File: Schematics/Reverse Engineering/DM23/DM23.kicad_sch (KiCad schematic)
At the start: 100 parts, among them J1 Conn_01x40, Q1 2N1499A, Q2 2N1499A, Q3 2N1499A, Q4 2N1499A, Q5 2N1499A, Q6 2N1499A, Q7 2N1499A, Q8 2N1499A, Q9 2N1499A

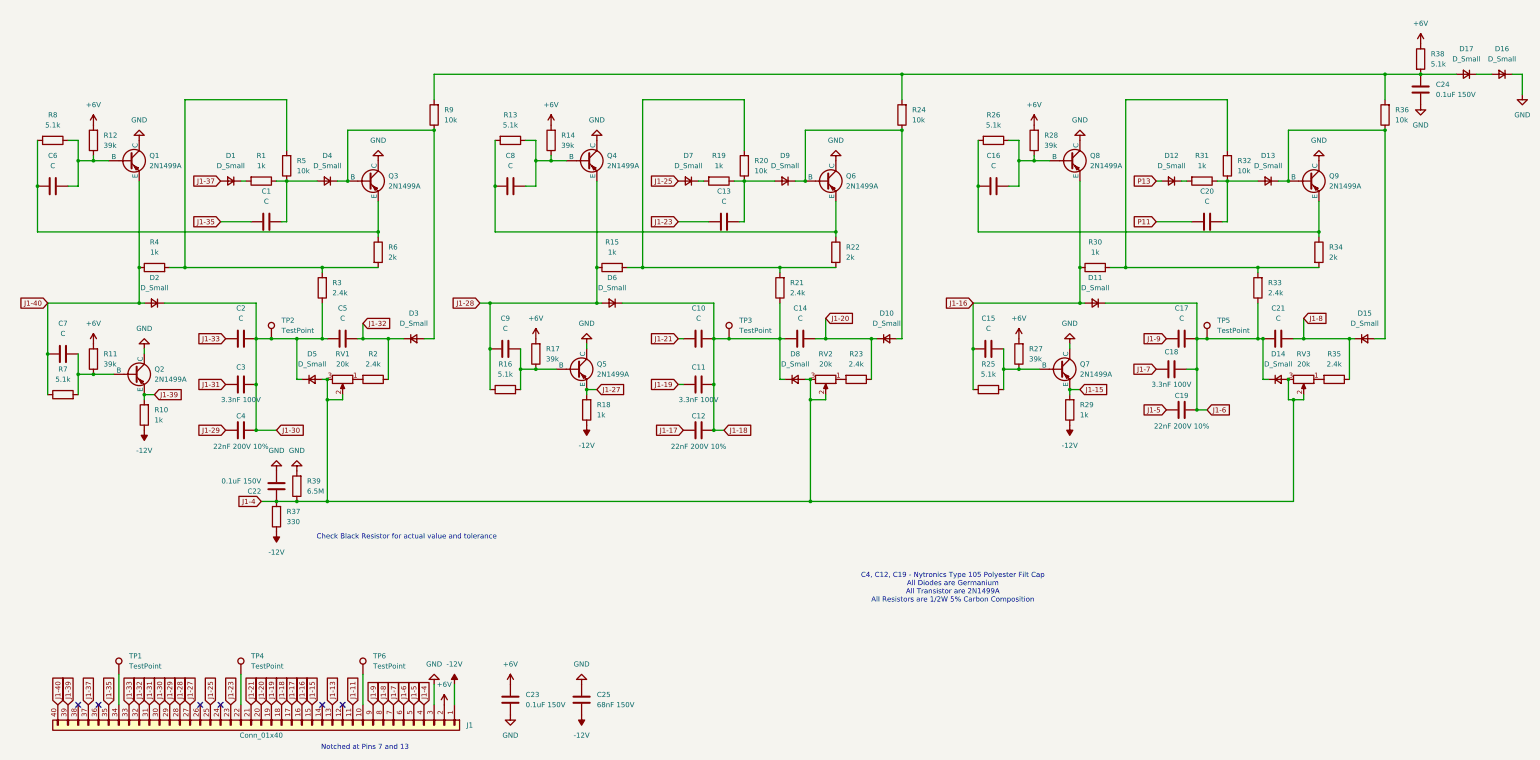
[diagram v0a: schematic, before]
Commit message: Updated Schematic Layout and PCB
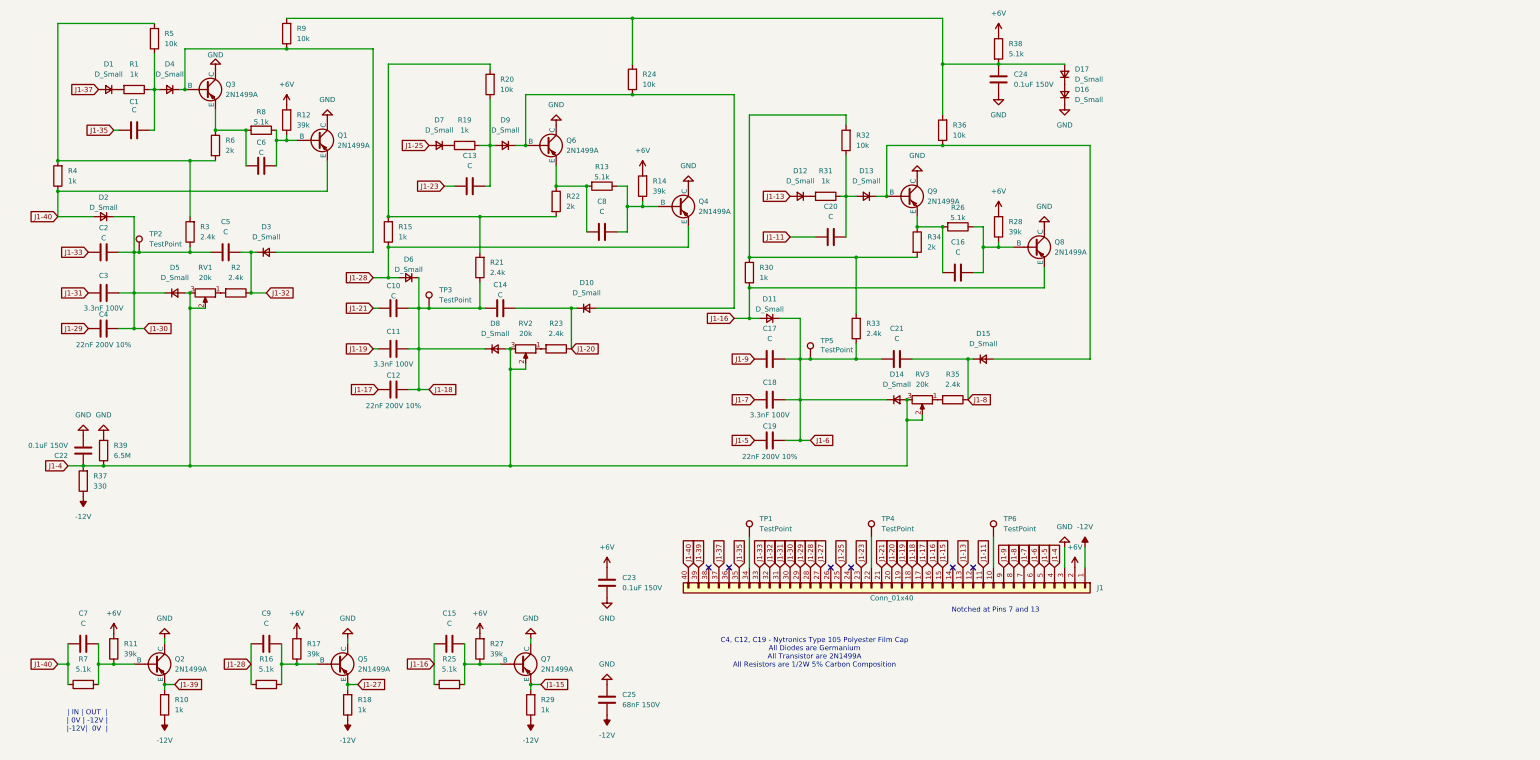
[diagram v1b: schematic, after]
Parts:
- R39: footprint (none) -> Resistor_THT:R_Axial_DIN0207_L6.3mm_D2.5mm_P10.16mm_Horizontal
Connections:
- net P11 is gone; now on net J1-11: C20.1
- net P13 is gone; now on net J1-13: D12.2 (A)
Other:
- note added: "C4, C12, C19 - Nytronics Type 105 Polyester Film Cap All Diodes are Germanium All Transistor are 2N1499A All Resistors are 1/2W 5% Carbon Composition"
- note added: "| IN | OUT | | 0V | -12V | |-12V| 0V |"
- note removed: "C4, C12, C19 - Nytronics Type 105 Polyester Filt Cap All Diodes are Germanium All Transistor are 2N1499A All Resistors are 1/2W 5% Carbon Composition"
- note removed: "Check Black Resistor for actual value and tolerance"
- moved on the sheet: C1, C10, C11, C12, C13, C14, C15, C16, C17, C18, C19, C2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

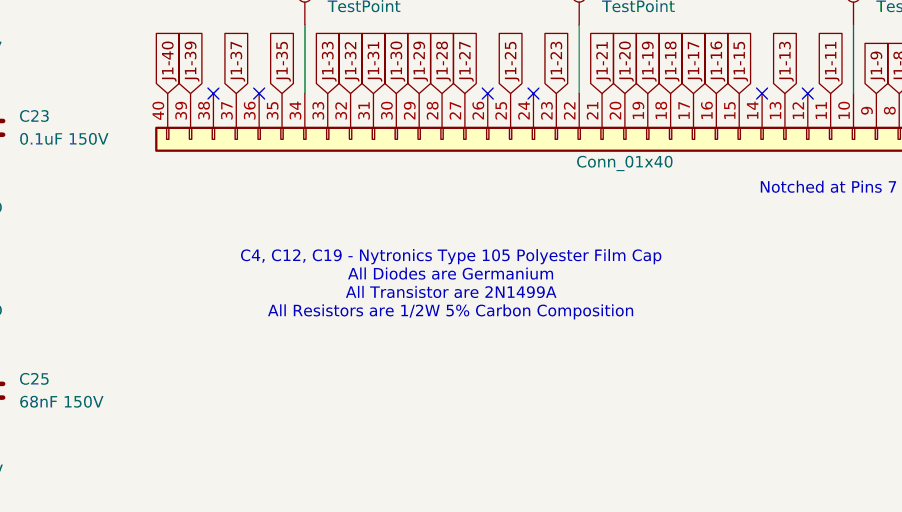
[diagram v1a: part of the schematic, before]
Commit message: LR312 Schematic and PCB
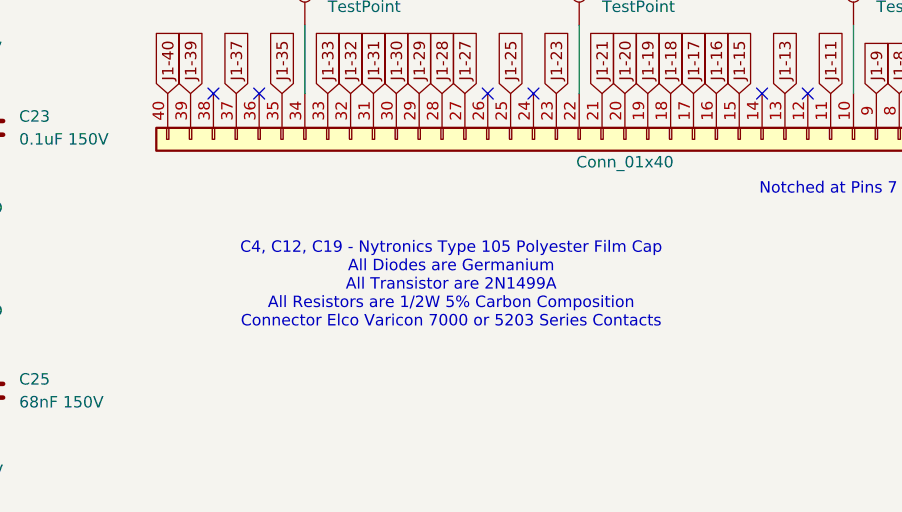
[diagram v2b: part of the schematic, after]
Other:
- note added: "C4, C12, C19 - Nytronics Type 105 Polyester Film Cap All Diodes are Germanium All Transistor are 2N1499A All Resistors are 1/2W 5% Carbon Composition Connector Elco Varicon 7000 or 5203 Series Contacts"
- note removed: "C4, C12, C19 - Nytronics Type 105 Polyester Film Cap All Diodes are Germanium All Transistor are 2N1499A All Resistors are 1/2W 5% Carbon Composition"
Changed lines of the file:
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@@
 		)
 	)
-	(text "C4, C12, C19 - Nytronics Type 105 Polyester Film Cap\nAll Diodes are Germanium\nAll Transistor are 2N1499A\nAll Resistors are 1/2W 5% Carbon Composition "
+	(text "C4, C12, C19 - Nytronics Type 105 Polyester Film Cap\nAll Diodes are Germanium\nAll Transistor are 2N1499A\nAll Resistors are 1/2W 5% Carbon Composition \nConnector Elco Varicon 7000 or 5203 Series Contacts"
 		(exclude_from_sim no)
 		(at 211.836 173.736 0)
